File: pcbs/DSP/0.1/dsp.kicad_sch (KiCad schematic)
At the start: 48 parts, among them J1 Conn_01x04_Pin, J10 Conn_01x04_Pin, J11 Conn_01x02_Pin, J2 Conn_01x03_Pin, J3 Conn_01x04_Pin, J4 Conn_01x04_Pin, J6 Conn_02x03_Odd_Even, J7 Conn_01x06_Pin, J8 Conn_01x02_Pin, J9 Conn_01x06_Pin, U1 ESP32-S3-WROOM-1, U2 ESP32-S3-WROOM-1, U3 PI6CV304, U4 PI6CV304, U5 PI6CV304, U6 ESP32-S3-WROOM-1

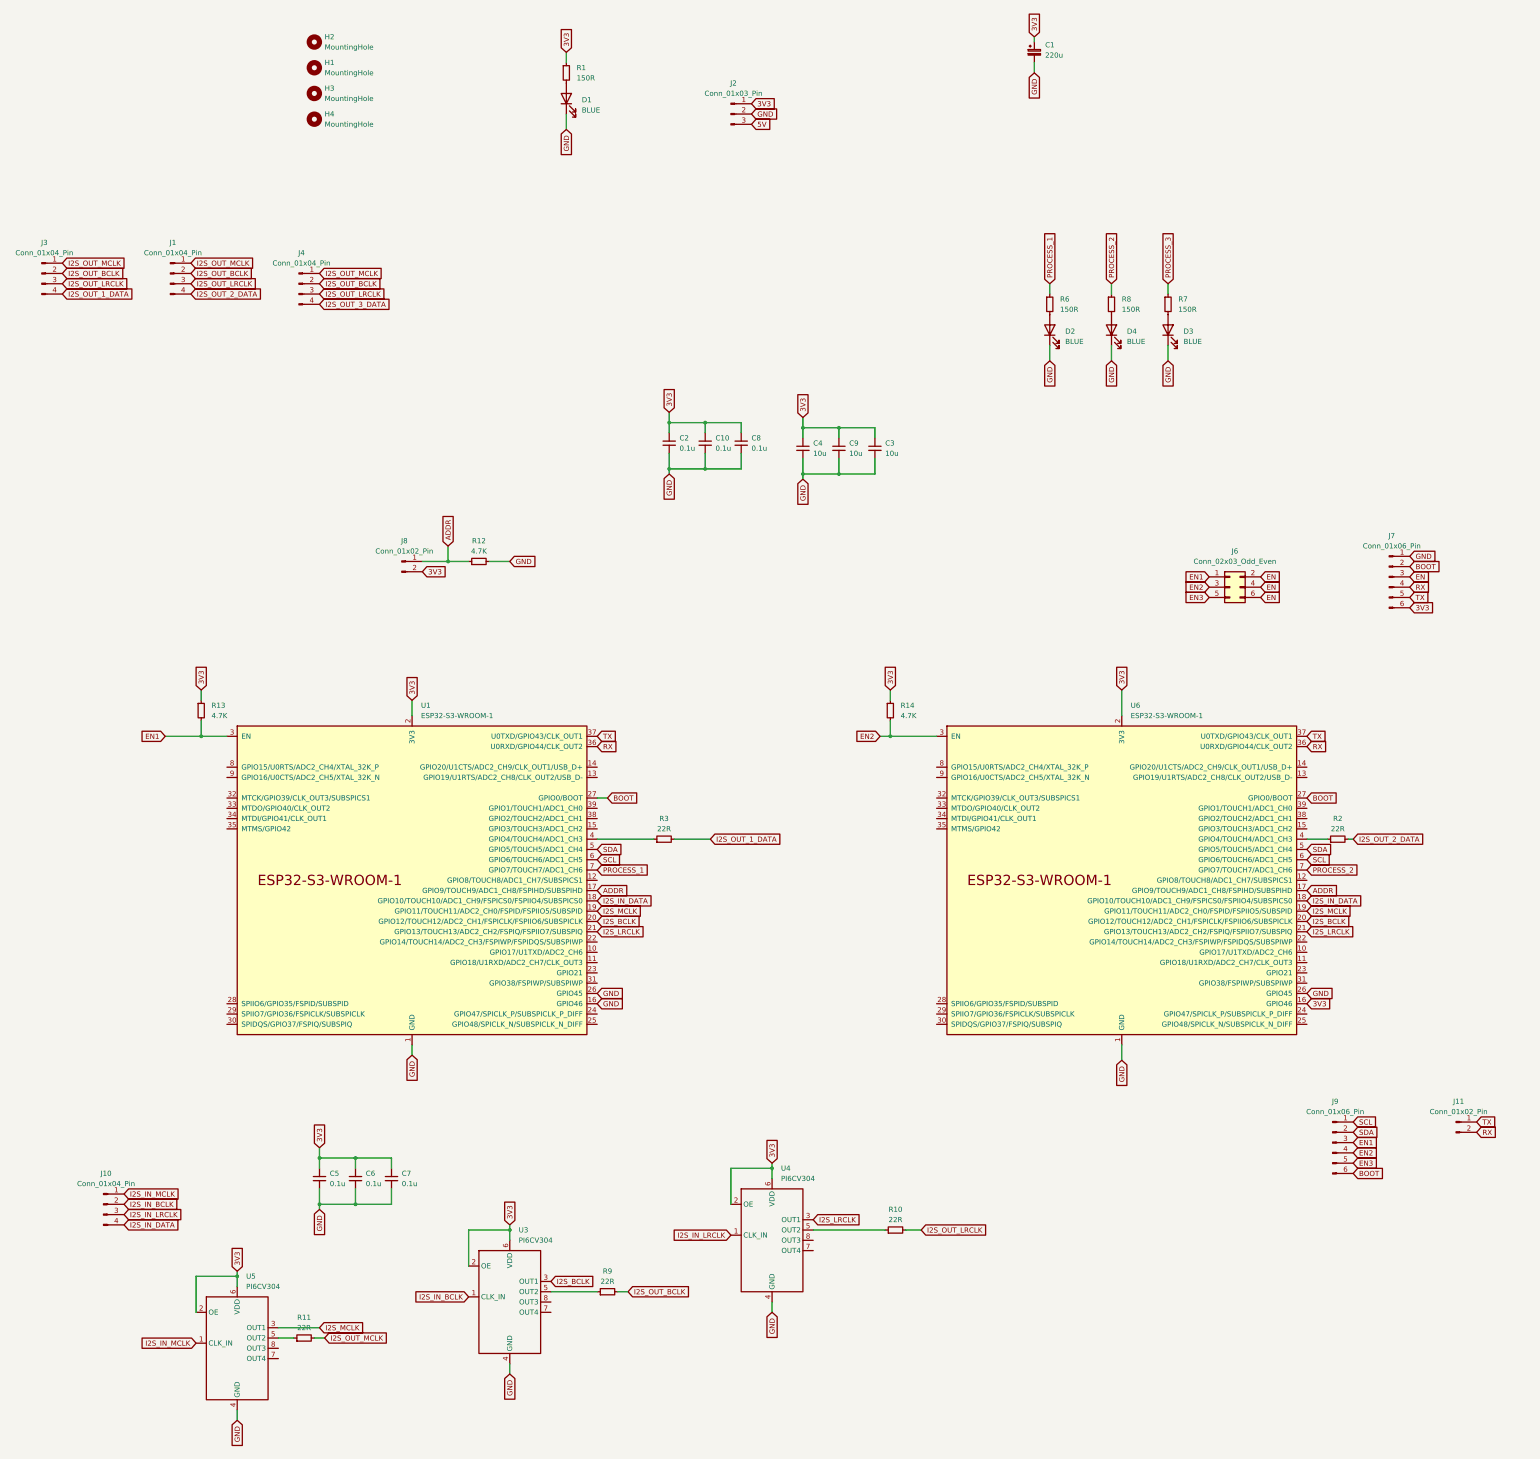
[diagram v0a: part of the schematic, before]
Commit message: Updates
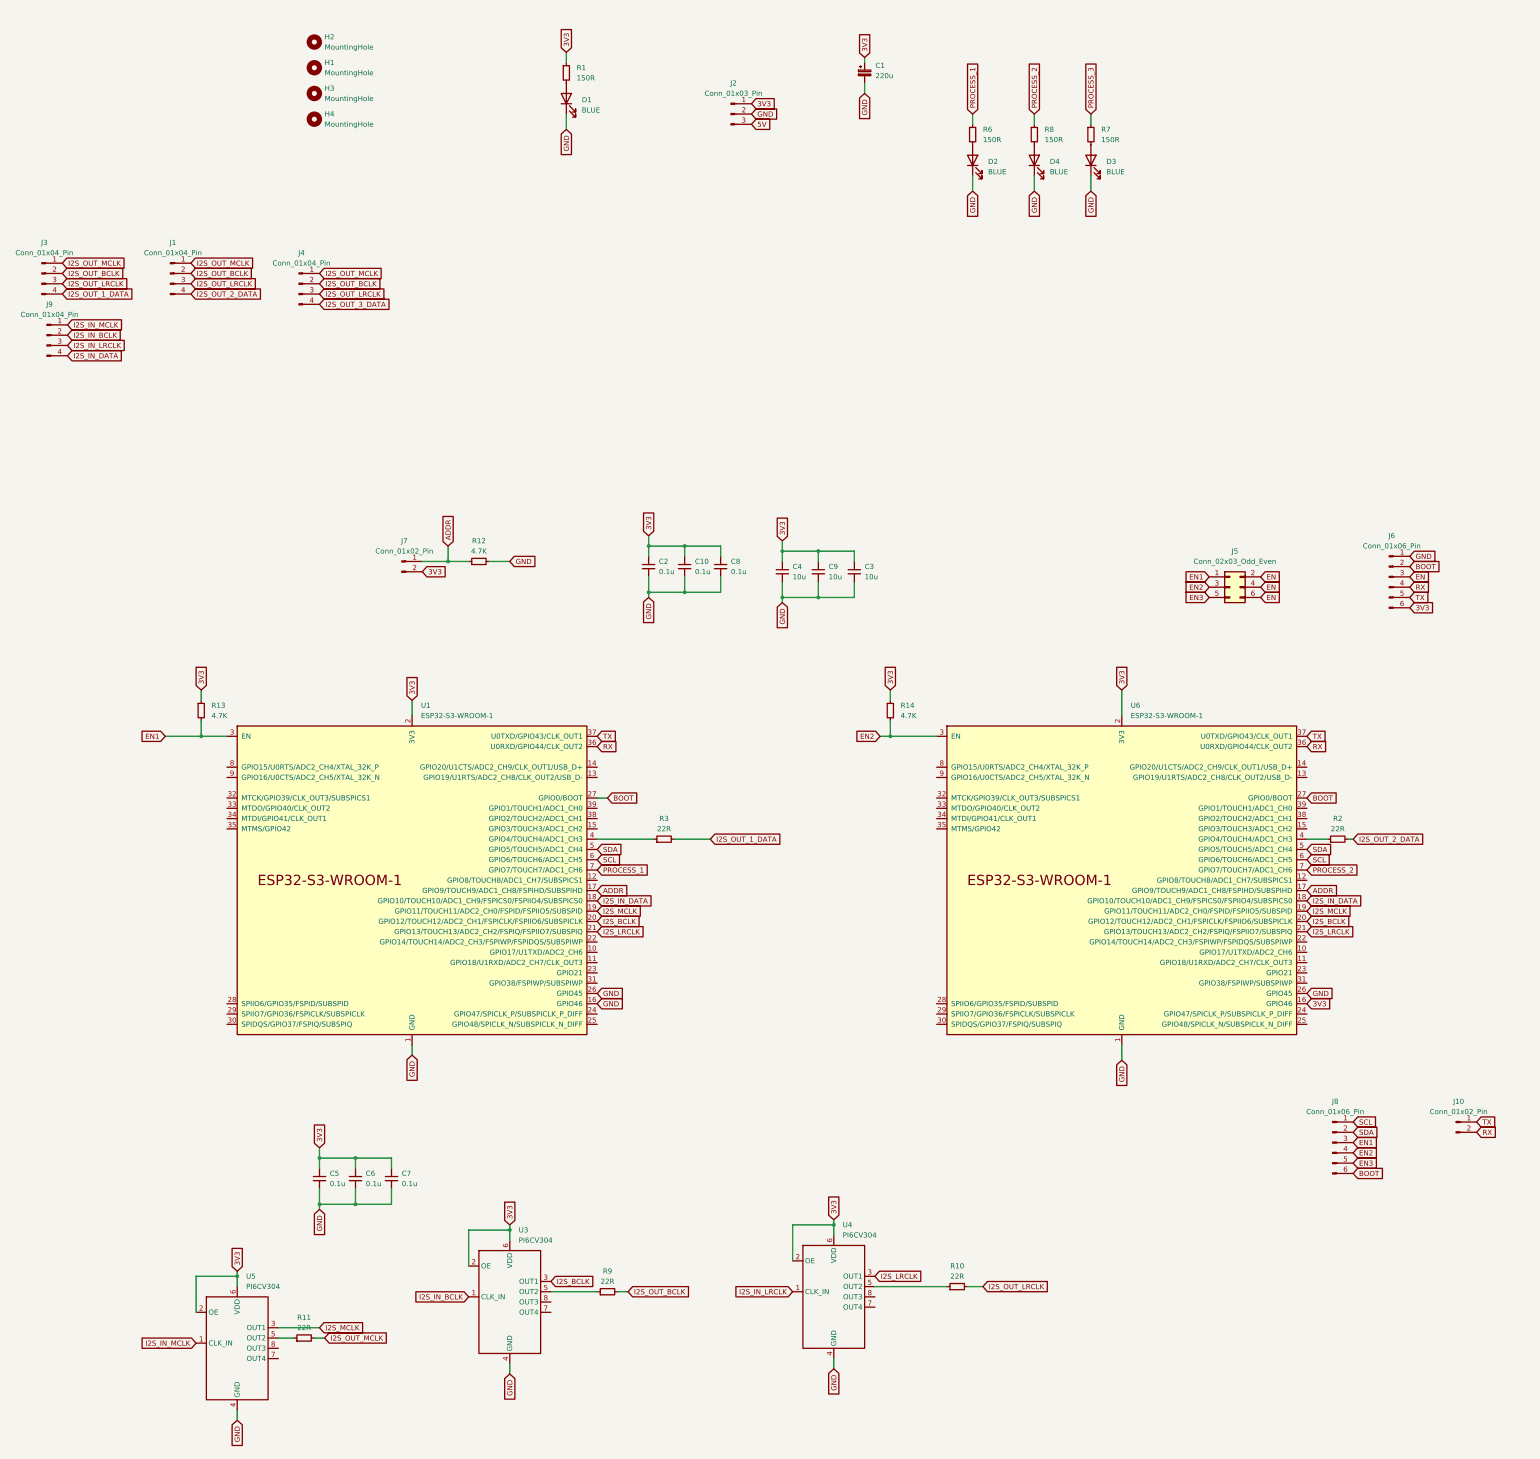
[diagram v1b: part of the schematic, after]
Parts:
- renumbered J11 to J10, J6 to J5, J7 to J6, J8 to J7, J9 to J8, J10 to J9
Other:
- moved on the sheet: C1, C10, C2, C3, C4, C8, C9, D2, D3, D4, J9, R10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
